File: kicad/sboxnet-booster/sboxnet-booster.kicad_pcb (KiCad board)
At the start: 2 copper layers, 70 parts, among them J1 sboxnet-stecker_02x17, J3 Conn_01x02_Male, J4 Conn_01x02_Male, J5 Screw_Terminal_01x04, J6 Screw_Terminal_01x04, J7 Power von externen 15V/4A Net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, SW1 Öffner, U1 L6206PSO-sboxnet, U2 L78L12_SOT89

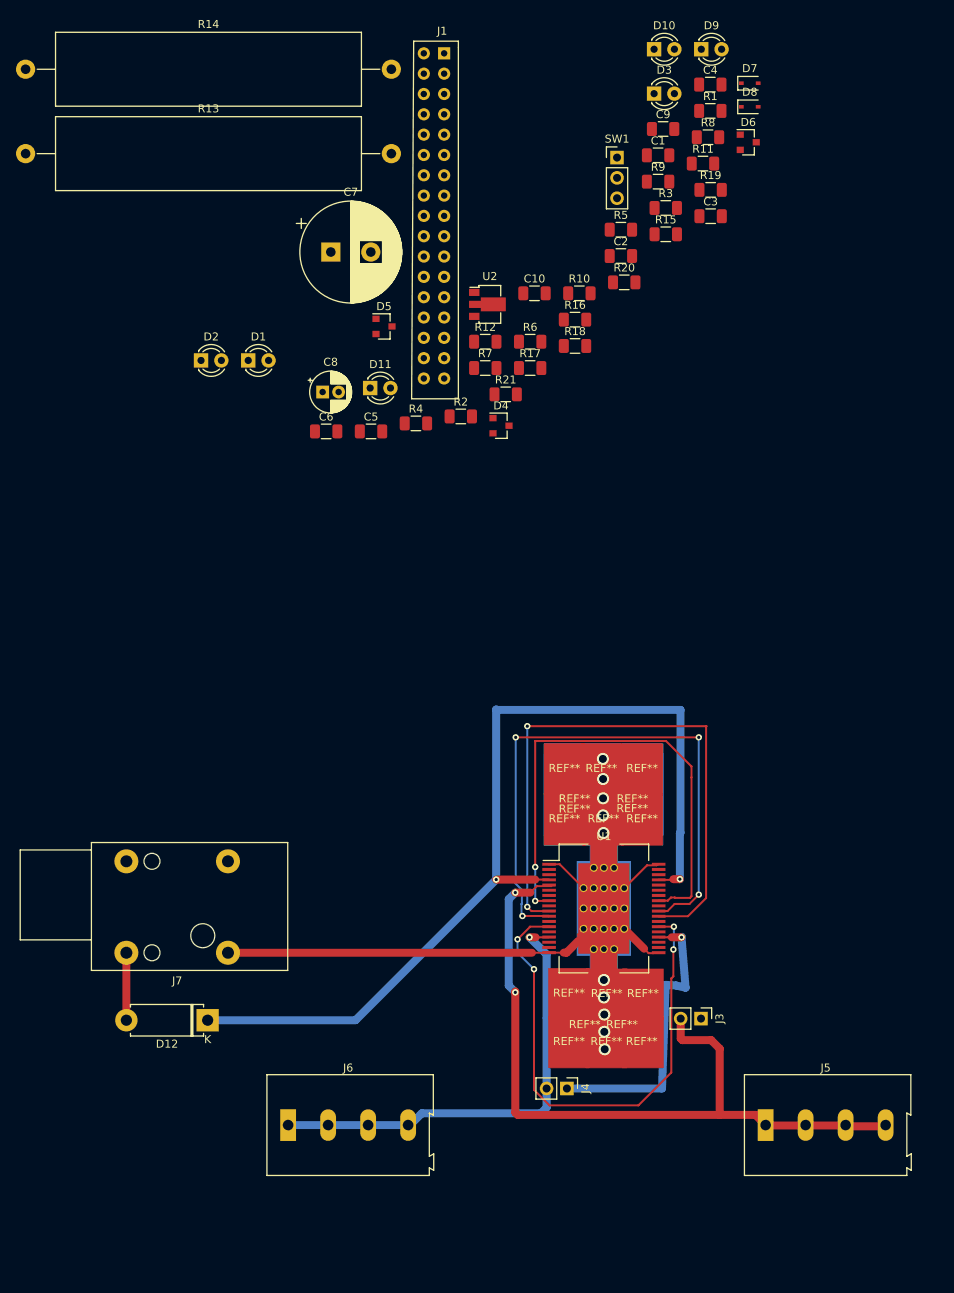
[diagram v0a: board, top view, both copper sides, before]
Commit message: work in progress layout
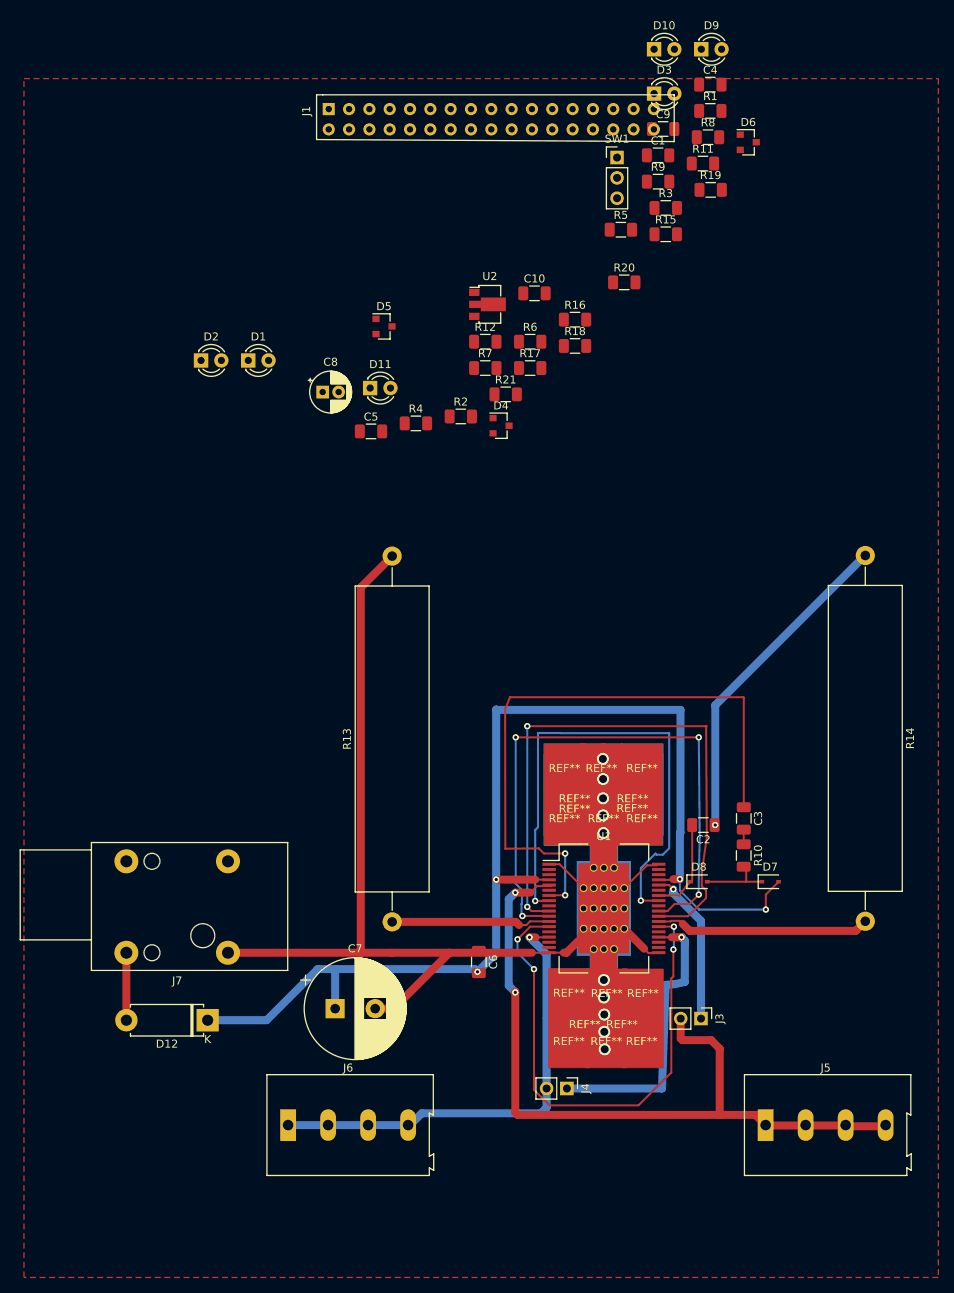
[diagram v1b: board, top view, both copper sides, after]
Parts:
- J7: value Power von externen 15V/4A Netzteil -> Power von externen 15V/4A Netzteil DS_NRJ4HF
- moved R14 121.3 mm to (130.6, 85.0), turned to 270 degrees
- moved R13 106.4 mm to (71.4, 130.8), turned to 90 degrees
- moved D7 99.8 mm to (118.7, 125.8)
- moved D8 97.1 mm to (109.8, 125.8)
- moved C7 94.6 mm to (64.3, 141.7)
- moved C3 75.4 mm to (115.4, 117.9), turned to 270 degrees
- moved R10 73.2 mm to (115.4, 122.5), turned to 270 degrees
- moved C2 71.9 mm to (110.3, 118.7), turned to 180 degrees
- moved C6 69.0 mm to (82.3, 135.8), turned to 270 degrees
- moved J1 18.8 mm to (61.0, 31.8), turned to 90 degrees
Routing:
- net GND: track 107.2 -> 211.7 mm, vias 0 -> 1
- net VCP: track 0.00 -> 76.9 mm, vias 0 -> 2
- net V: track 118.1 -> 146.1 mm, vias 2 -> 4
- net Net-(R14-Pad2): track 0.00 -> 26.9 mm
- net OUT2b: track 0.00 -> 19.9 mm, vias 0 -> 1
- net Net-(R13-Pad1): track 0.00 -> 19.3 mm
- net VBOOT: track 0.00 -> 11.8 mm
- net Net-(D7-Pad1): track 0.00 -> 8.84 mm
- net Net-(C3-Pad2): track 0.00 -> 1.87 mm
- net EN: track 63.2 -> 64.7 mm
- net OUT1b: track 36.6 -> 35.9 mm
- added copper zone on F.Cu, net GND
